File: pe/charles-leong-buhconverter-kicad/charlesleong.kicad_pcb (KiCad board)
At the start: 2 copper layers, 9 parts, among them U1 TPS542025DDCR

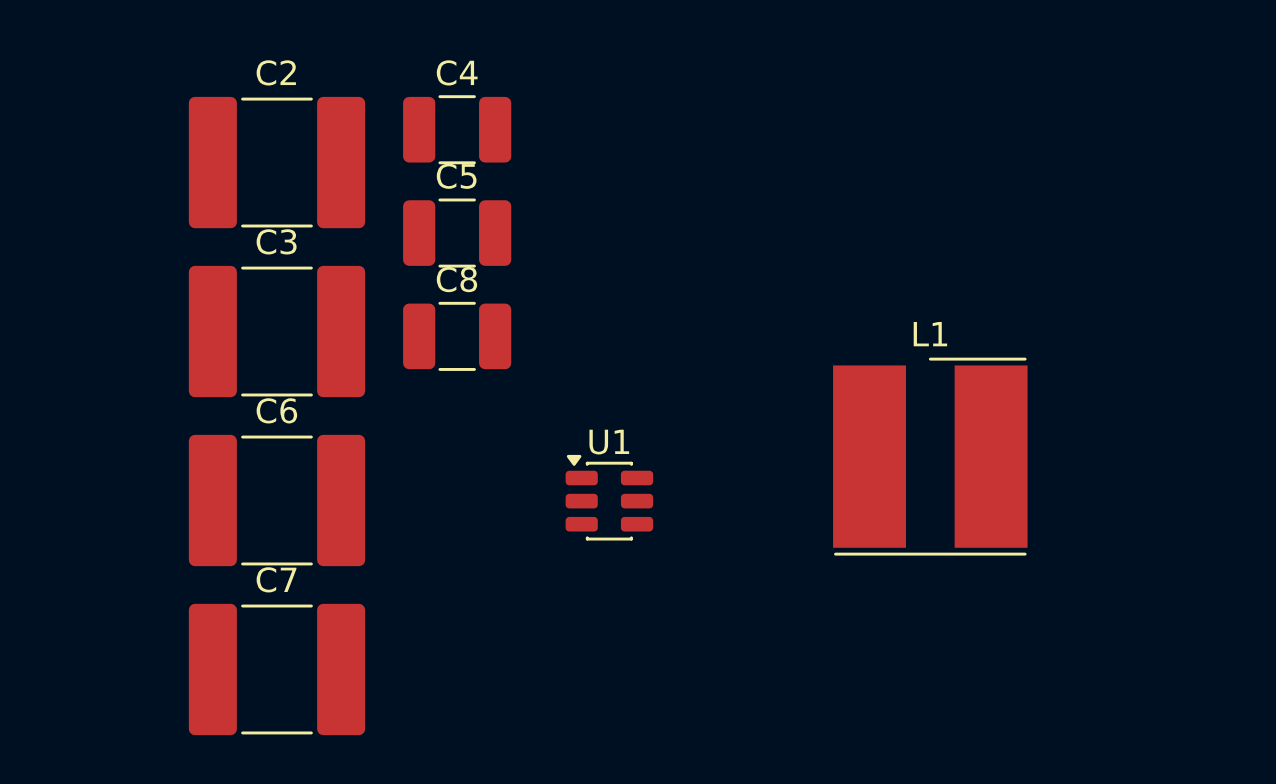
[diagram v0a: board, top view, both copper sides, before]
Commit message: pcb components
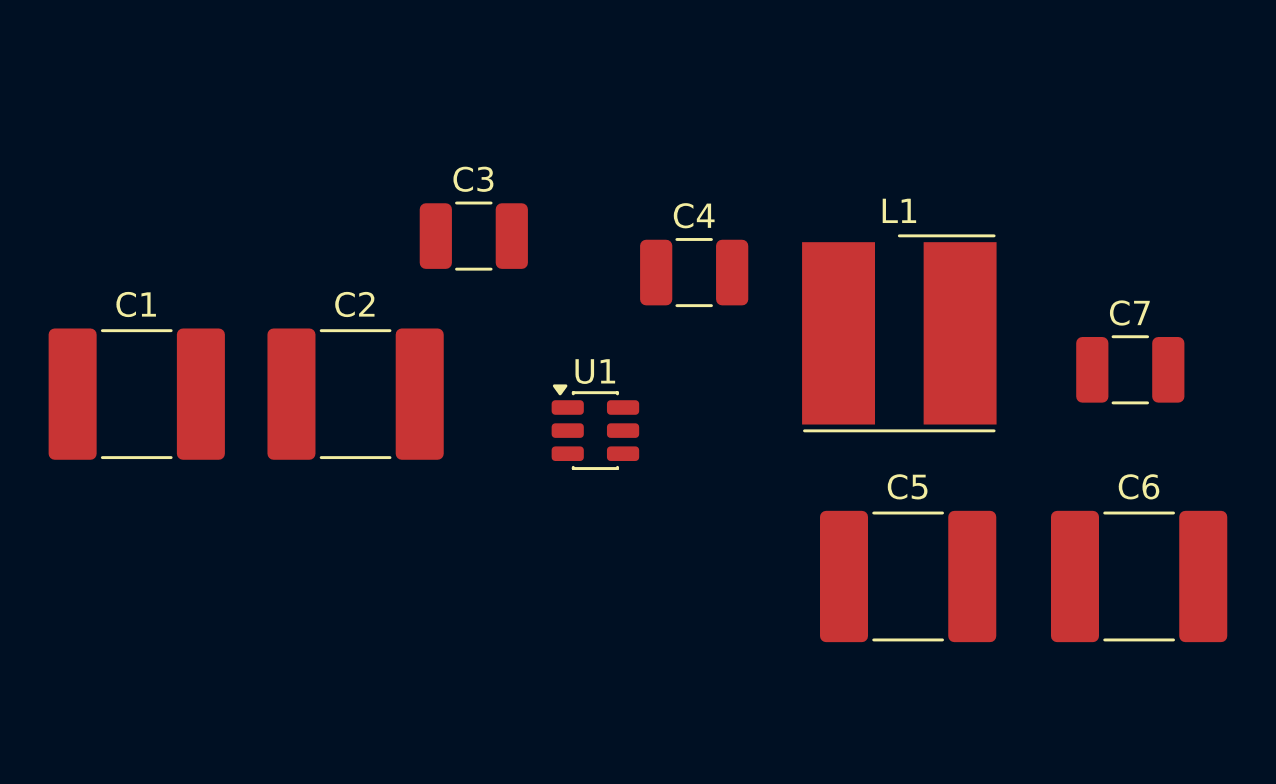
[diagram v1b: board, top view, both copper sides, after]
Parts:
- moved C6 35.7 mm to (141.4, 79.0)
- moved C7 27.7 mm to (141.0, 70.5)
- moved C5 26.1 mm to (131.9, 79.0)
- moved C1 11.1 mm to (100.1, 71.5)
- moved C4 9.88 mm to (123.1, 66.5)
- moved L1 5.23 mm to (131.5, 69.0)
- moved C3 4.43 mm to (114.0, 65.0)
- moved C2 4.13 mm to (109.1, 71.5)
- moved U1 2.96 mm to (119.0, 73.0)
- renumbered C2 to C1, C3 to C2, C4 to C3, C5 to C4, C6 to C5, C7 to C6, C8 to C7
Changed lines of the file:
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@@
 		(capping no)
 		(filling no)
+		(zone_defaults)
 		(pcbplotparams
 			(layerselection 0x00000000_00000000_55555555_5755f5ff)
@@
 	(footprint "Capacitor_SMD:C_2220_5750Metric_Pad1.97x5.40mm_HandSolder"
 		(layer "F.Cu")
-		(at 105.905 82.825)
+		(at 141.3625 79)
 		(descr "Capacitor SMD 2220 (5750 Metric), square (rectangular) end terminal, IPC-7351 nominal with elongated pad for handsoldering. (Body size from: http://datasheets.avx.com/AVX-HV_MLCC.pdf)")
 		(tags "capacitor handsolder")
-		(property "Reference" "C7"
+		(property "Reference" "C6"
 			(at 0 -3.65 0)
 			(layer "F.SilkS")
@@
 	(footprint "Capacitor_SMD:C_1210_3225Metric_Pad1.33x2.70mm_HandSolder"
 		(layer "F.Cu")
-		(at 113.315 69.125)
+		(at 141 70.5)
 		(descr "Capacitor SMD 1210 (3225 Metric), square (rectangular) end terminal, IPC-7351 nominal with elongated pad for handsoldering. (Body size source: IPC-SM-782 page 76, https://www.pcb-3d.com/wordpress/wp-content/uploads/ipc-sm-782a_amendment_1_and_2.pdf)")
 		(tags "capacitor handsolder")
-		(property "Reference" "C8"
+		(property "Reference" "C7"
 			(at 0 -2.3 0)
 			(layer "F.SilkS")
@@
 	(footprint "Package_TO_SOT_SMD:SOT-23-6"
 		(layer "F.Cu")
-		(at 119.575 75.9)
+		(at 119 73)
 		(descr "SOT, 6 Pin (JEDEC MO-178 Var AB https://www.jedec.org/document_search?search_api_views_fulltext=MO-178)")
 		(tags "SOT TO_SOT_SMD")
@@
 	(footprint "Capacitor_SMD:C_1210_3225Metric_Pad1.33x2.70mm_HandSolder"
 		(layer "F.Cu")
-		(at 113.315 64.875)
+		(at 123.0625 66.5)
 		(descr "Capacitor SMD 1210 (3225 Metric), square (rectangular) end terminal, IPC-7351 nominal with elongated pad for handsoldering. (Body size source: IPC-SM-782 page 76, https://www.pcb-3d.com/wordpress/wp-content/uploads/ipc-sm-782a_amendment_1_and_2.pdf)")
 		(tags "capacitor handsolder")
-		(property "Reference" "C5"
+		(property "Reference" "C4"
 			(at 0 -2.3 0)
 			(layer "F.SilkS")
@@
 	(footprint "Capacitor_SMD:C_2220_5750Metric_Pad1.97x5.40mm_HandSolder"
 		(layer "F.Cu")
-		(at 105.905 75.875)
+		(at 131.8625 79)
 		(descr "Capacitor SMD 2220 (5750 Metric), square (rectangular) end terminal, IPC-7351 nominal with elongated pad for handsoldering. (Body size from: http://datasheets.avx.com/AVX-HV_MLCC.pdf)")
 		(tags "capacitor handsolder")
-		(property "Reference" "C6"
+		(property "Reference" "C5"
 			(at 0 -3.65 0)
 			(layer "F.SilkS")
@@
 	(footprint "formula_slug_footprint_library:L_Wurth_WE-PD2SR-7850"
 		(layer "F.Cu")
-		(at 132.775 74.07)
+		(at 131.5 69)
 		(descr "Shielded Power Inductor, body 7.8x7x5mm, https://www.we-online.com/en/components/products/WE-PD2SR#/articles/WE-PD2SR-7850")
 		(tags "SMT")
@@
 	(footprint "Capacitor_SMD:C_2220_5750Metric_Pad1.97x5.40mm_HandSolder"
 		(layer "F.Cu")
-		(at 105.905 68.925)
+		(at 109.1375 71.5)
 		(descr "Capacitor SMD 2220 (5750 Metric), square (rectangular) end terminal, IPC-7351 nominal with elongated pad for handsoldering. (Body size from: http://datasheets.avx.com/AVX-HV_MLCC.pdf)")
 		(tags "capacitor handsolder")
-		(property "Reference" "C3"
+		(property "Reference" "C2"
 			(at 0 -3.65 0)
 			(layer "F.SilkS")
@@
 	(footprint "Capacitor_SMD:C_2220_5750Metric_Pad1.97x5.40mm_HandSolder"
 		(layer "F.Cu")
-		(at 105.905 61.975)
+		(at 100.1375 71.5)
 		(descr "Capacitor SMD 2220 (5750 Metric), square (rectangular) end terminal, IPC-7351 nominal with elongated pad for handsoldering. (Body size from: http://datasheets.avx.com/AVX-HV_MLCC.pdf)")
 		(tags "capacitor handsolder")
-		(property "Reference" "C2"
+		(property "Reference" "C1"
 			(at 0 -3.65 0)
 			(layer "F.SilkS")
@@
 	(footprint "Capacitor_SMD:C_1210_3225Metric_Pad1.33x2.70mm_HandSolder"
 		(layer "F.Cu")
-		(at 113.315 60.625)
+		(at 114 65)
 		(descr "Capacitor SMD 1210 (3225 Metric), square (rectangular) end terminal, IPC-7351 nominal with elongated pad for handsoldering. (Body size source: IPC-SM-782 page 76, https://www.pcb-3d.com/wordpress/wp-content/uploads/ipc-sm-782a_amendment_1_and_2.pdf)")
 		(tags "capacitor handsolder")
-		(property "Reference" "C4"
+		(property "Reference" "C3"
 			(at 0 -2.3 0)
 			(layer "F.SilkS")

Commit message: aligning pcb components
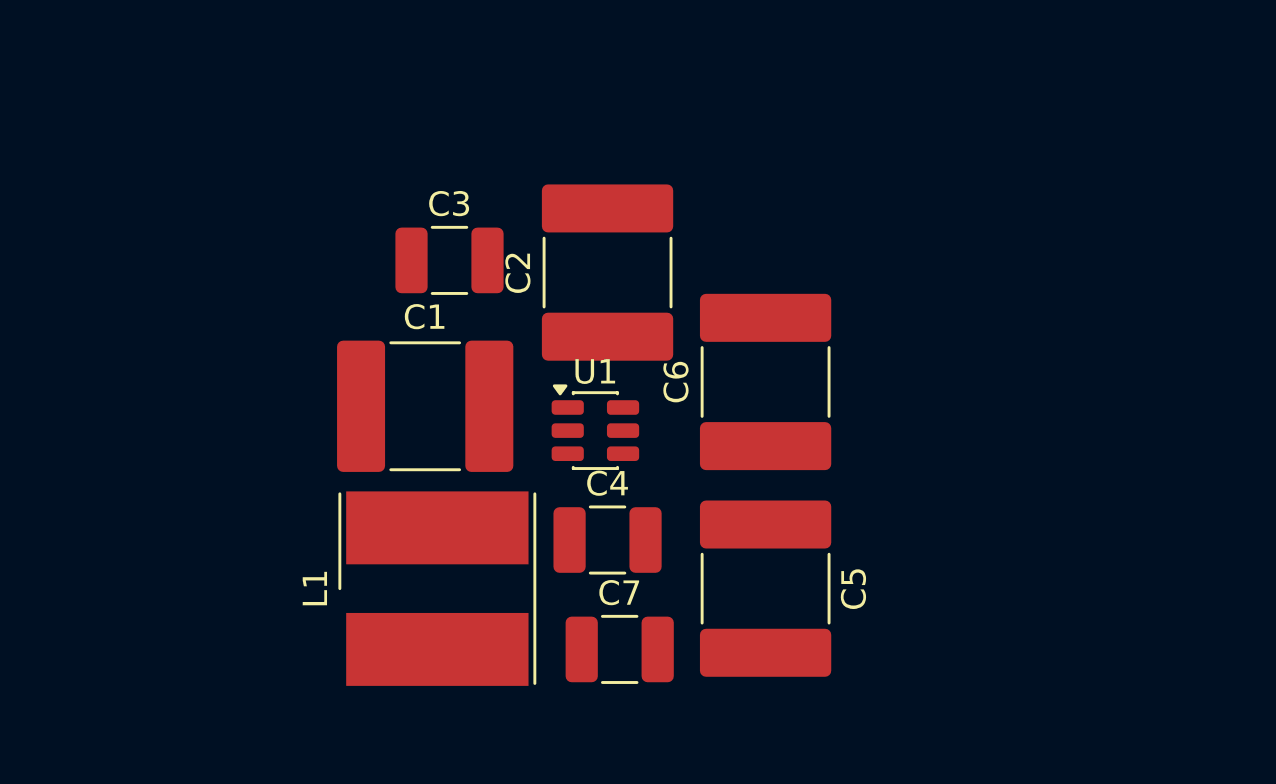
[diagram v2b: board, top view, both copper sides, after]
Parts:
- moved C7 23.9 mm to (120.0, 82.0)
- moved L1 21.7 mm to (112.5, 79.5), turned to 90 degrees
- moved C6 17.3 mm to (126.0, 71.0), turned to 90 degrees
- moved C1 11.9 mm to (112.0, 72.0)
- moved C4 11.6 mm to (119.5, 77.5)
- moved C2 11.5 mm to (119.5, 66.5), turned to 90 degrees
- moved C5 5.88 mm to (126.0, 79.5), turned to -90 degrees
- moved C3 1.41 mm to (113.0, 66.0)
